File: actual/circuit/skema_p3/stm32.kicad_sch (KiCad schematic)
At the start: 1 part

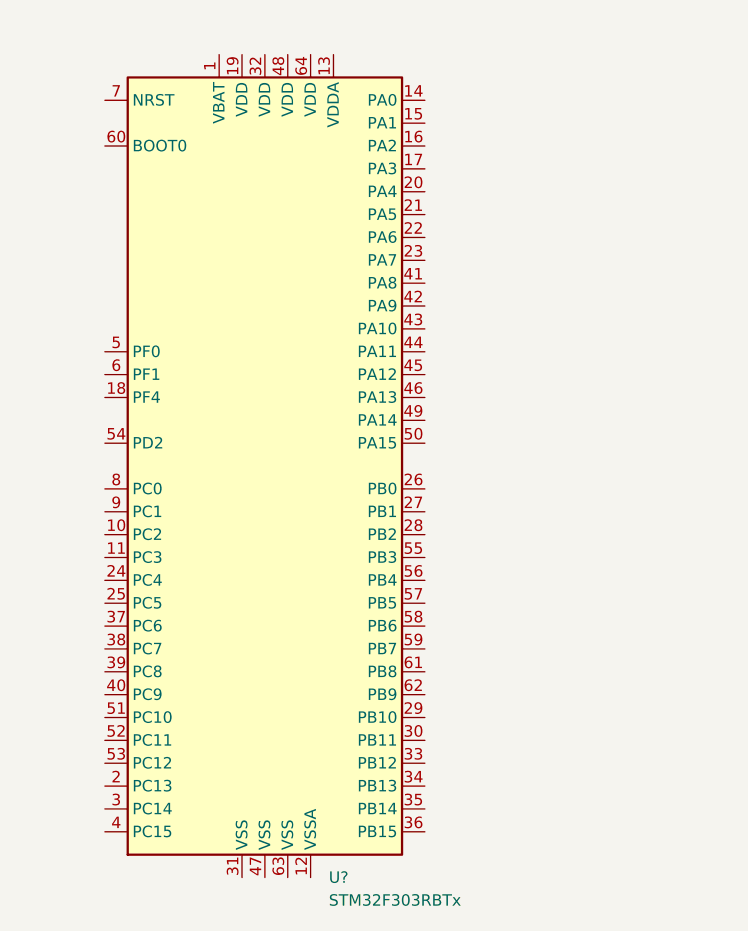
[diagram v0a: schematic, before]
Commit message: P3 in KiCAD
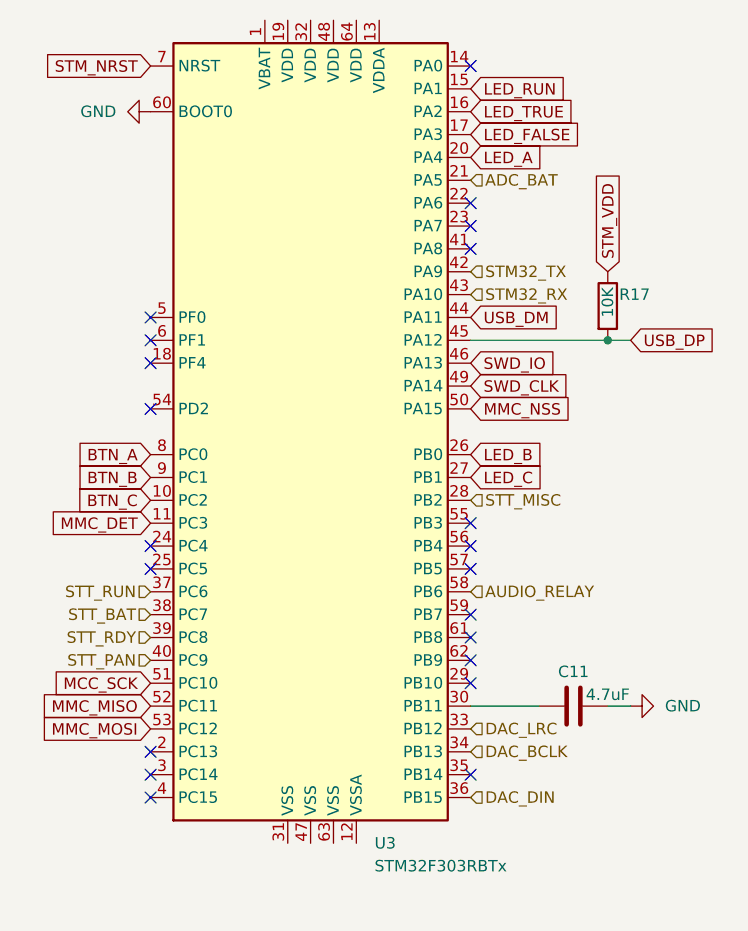
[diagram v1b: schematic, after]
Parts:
- added C11: 4.7uF, symbol Device:C
- added R17: 10K, symbol Device:R
- gave numbers to parts that had none: 1
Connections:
- net BTN_C: now reaches U3.10 (PC2)
- net MMC_DET: now reaches U3.11 (PC3)
- net LED_RUN: now reaches U3.15 (PA1)
- net LED_TRUE: now reaches U3.16 (PA2)
- net LED_FALSE: now reaches U3.17 (PA3)
- net LED_A: now reaches U3.20 (PA4)
- net ADC_BAT: now reaches U3.21 (PA5)
- net LED_B: now reaches U3.26 (PB0)
- net LED_C: now reaches U3.27 (PB1)
- net STT_MISC: now reaches U3.28 (PB2)
- net at U3.30 (PB11): now also C11.1
- net DAC_LRC: now reaches U3.33 (PB12)
- net DAC_BCLK: now reaches U3.34 (PB13)
- net DAC_DIN: now reaches U3.36 (PB15)
- net STT_RUN: now reaches U3.37 (PC6)
- net STT_BAT: now reaches U3.38 (PC7)
- net STT_RDY: now reaches U3.39 (PC8)
- net STT_PAN: now reaches U3.40 (PC9)
- net STM32_TX: now reaches U3.42 (PA9)
- net STM32_RX: now reaches U3.43 (PA10)
- net USB_DM: now reaches U3.44 (PA11)
- net USB_DP: now reaches U3.45 (PA12)
- net USB_DP: now also R17.2
- net SWD_IO: now reaches U3.46 (PA13)
- net SWD_CLK: now reaches U3.49 (PA14)
- net MMC_NSS: now reaches U3.50 (PA15)
- net MCC_SCK: now reaches U3.51 (PC10)
- net MMC_MISO: now reaches U3.52 (PC11)
- net MMC_MOSI: now reaches U3.53 (PC12)
- net AUDIO_RELAY: now reaches U3.58 (PB6)
- net GND: now reaches U3.60 (BOOT0)
- net GND: now also C11.2
- net STM_NRST: now reaches U3.7 (NRST)
- net BTN_A: now reaches U3.8 (PC0)
- net BTN_B: now reaches U3.9 (PC1)
- new net STM_VDD: R17.1
- no-connect marks 0 -> 21
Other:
- moved on the sheet: U3
